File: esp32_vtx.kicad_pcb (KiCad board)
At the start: 4 copper layers, 20.1 x 23.3 mm, 38 parts, among them J1 Conn_01x24_MountingPin, J2 Conn_01x04, SW1 SW_SPST, SW2 SW_SPST, U1 AMS1117-3.3, U2 IS25WP032, U3 ESP32-PICO-D4, U4 MKDV4GCL-AB, U5 XC6206-2.8V, U6 XC6206-1.2V

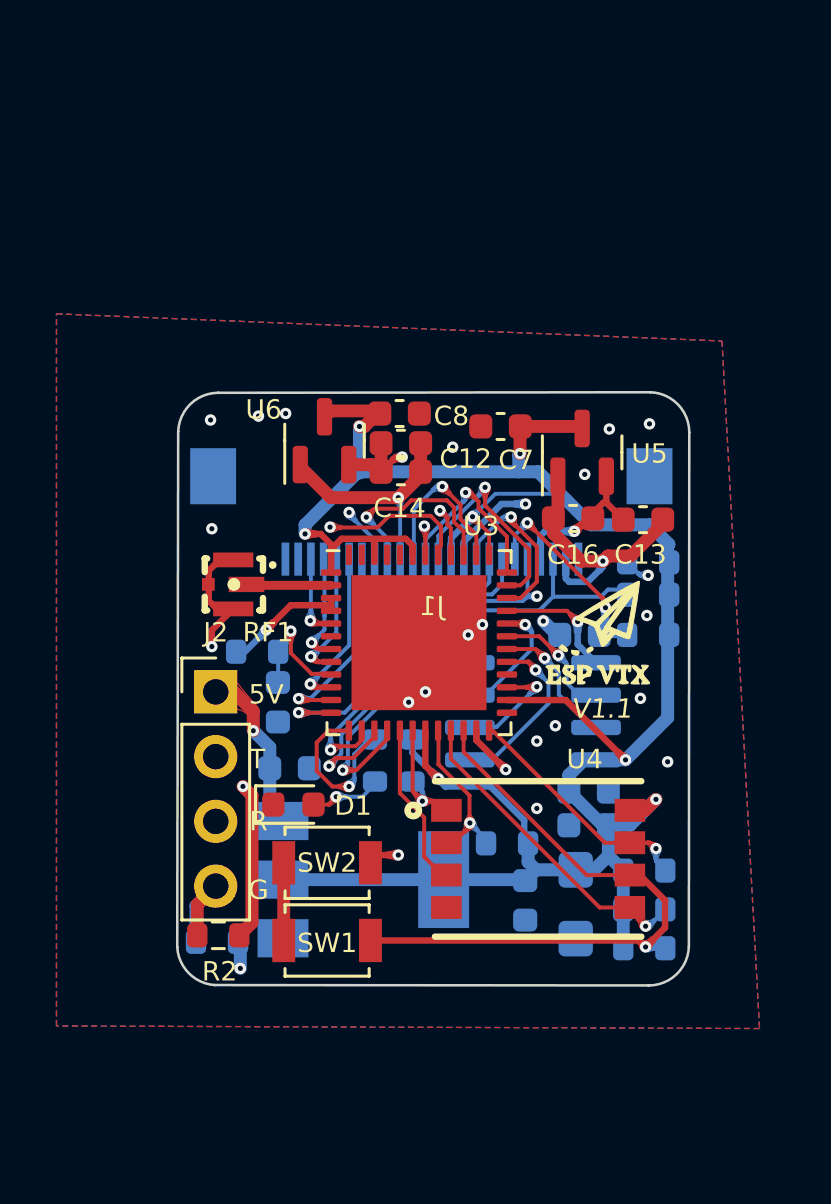
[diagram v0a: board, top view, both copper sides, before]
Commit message: update
Signed-off-by: huangzzk <huangcmzzk@gmail.com>
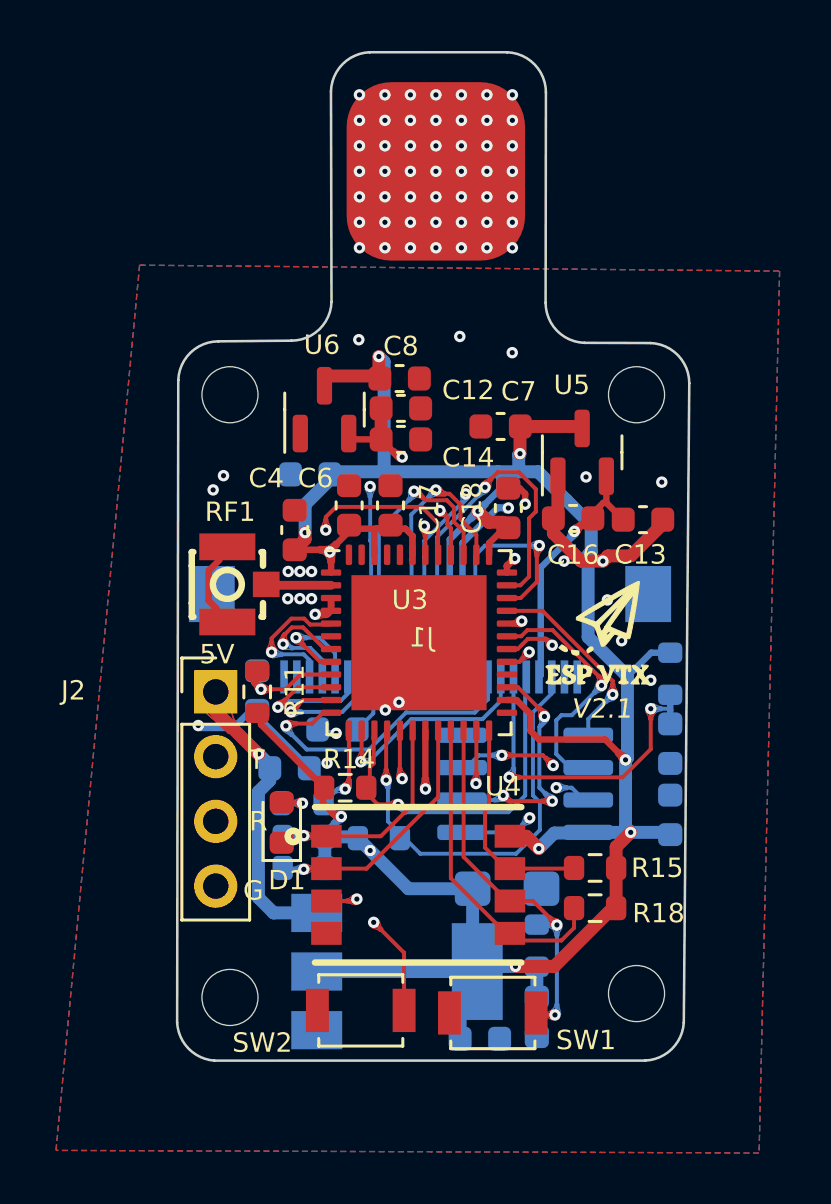
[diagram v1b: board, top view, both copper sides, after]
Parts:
- removed R2, R3: 0R, Resistor_SMD:R_0603_1608Metric
- added ?: , , F.Cu at (132.4, 78.9)
- added C17: 10u, Capacitor_SMD:C_0603_1608Metric, F.Cu at (130.7, 92.0)
- added C18: 10u, Capacitor_SMD:C_0603_1608Metric, F.Cu at (135.3, 92.2)
- added C19: 10u, Capacitor_SMD:C_0603_1608Metric, B.Cu at (127.5, 90.8)
- added C4: 10u, Capacitor_SMD:C_0603_1608Metric, F.Cu at (126.9, 93.0)
- added C6: 10u, Capacitor_SMD:C_0603_1608Metric, F.Cu at (129.0, 92.0)
- added H1: MountingHole, MountingHole:MountingHole_2.2mm_M2, F.Cu at (124.4, 111.4)
- added H2: MountingHole, MountingHole:MountingHole_2.2mm_M2, F.Cu at (124.4, 87.7)
- added H3: MountingHole, MountingHole:MountingHole_2.2mm_M2, F.Cu at (140.3, 111.2)
- added H4: MountingHole, MountingHole:MountingHole_2.2mm_M2, F.Cu at (140.3, 87.7)
- R11, R14, R15, R18: moved to F.Cu
- RF1: value KH-IPEX4-2020 -> BWIPX-1-001E; footprint ic_footprint:IPEX4-SMD_4P-L1.8-W1.7-LS2.0-L_KH-IPEX4-2020 -> kicad_lceda:IPEX-SMD_BWIPX-1-001E
- moved R14 14.8 mm to (128.9, 103.1), turned to 0 degrees
- moved R9 14.2 mm to (130.2, 105.1), turned to 0 degrees
- moved C15 9.41 mm to (134.2, 113.0), turned to 180 degrees
- moved R17 8.03 mm to (127.3, 106.3)
- moved SW1 7.10 mm to (134.7, 112.0)
- moved SW2 5.94 mm to (129.5, 111.9)
- moved C2 5.63 mm to (128.6, 100.8), turned to 180 degrees
- moved C9 5.55 mm to (141.6, 101.4), turned to -90 degrees
- moved R16 5.21 mm to (127.3, 105.1), turned to 180 degrees
- moved U4 4.82 mm to (131.7, 106.9)
- moved J1 4.62 mm to (132.2, 96.9)
- moved C5 4.59 mm to (136.4, 112.1)
- moved R13 4.22 mm to (136.4, 109.3), turned to 90 degrees
- moved U1 3.84 mm to (130.9, 110.3)
- moved C10 3.33 mm to (141.6, 104.2), turned to -90 degrees
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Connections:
- net /SD_DATA0 renamed /GPIO2
- C12 pad 2: GNDD -> GND
- C13 pad 2: GNDA -> GND
- C14 pad 2: GNDD -> GND
- C16 pad 2: GNDA -> GND
- C2 pad 2: GNDD -> GND
- J1 pad 10: GNDD -> GND
- J1 pad 23: GNDA -> GND
- U5 pad 1: GNDA -> GND
- U6 pad 1: GNDD -> GND
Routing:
- net GNDA: track 37.4 -> 0.00 mm, vias 2 -> 0
- net GNDD: track 31.7 -> 0.00 mm, vias 2 -> 0
- net +3V3: track 104.8 -> 121.8 mm, vias 8 -> 13
- net /GPIO2: track 24.5 -> 14.6 mm, vias 1 -> 2
- net /SIO2: track 4.25 -> 11.9 mm, vias 1 -> 3
- net /SCL: track 20.7 -> 13.7 mm, vias 3 -> 1
- net /D9: track 8.80 -> 15.3 mm
- net /PCLK: track 9.60 -> 15.5 mm
- net GND: track 12.6 -> 18.4 mm, vias 20 -> 24
- net /SO: track 3.73 -> 9.33 mm, vias 1 -> 3
- net /RESET: track 8.15 -> 13.5 mm
- net +5V: track 6.58 -> 11.7 mm
- net /MCLK: track 7.17 -> 12.1 mm, vias 1 -> 2
- net /GPIO0: track 8.40 -> 13.1 mm
- net /SCLK: track 4.22 -> 8.96 mm
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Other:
- board size 20.1 x 23.3 mm -> 20.1 x 39.6 mm
- board text added: "V2.1"
- board text removed: "V1.1"
